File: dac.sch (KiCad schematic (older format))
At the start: 21 parts, among them J1 RCJ-2121, J2 Conn_01x03_Male, SW1 SW_DIP_x01, U1 pcm5102a

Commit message: correcciones en el esquematico indicadas  por el profesor
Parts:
- J1: Número de cátalogo (none) -> CP-1430-ND
- SW1: Código de catálogo en Digikey. (none) -> EG5071-ND
- U1: Código de catálogo en Digikey. (none) -> 296-36705-2-ND
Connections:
- net labels added: FLT, GND, OUTL, OUTR
- net labels removed: Earth
- wire segments 81 -> 77
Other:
- note added: "Conexiones del CI"
- note added: "output circuit"
- moved on the sheet: C1, C10, C11, C12, C13, C2, C3, C4, C5, C6, C7, C8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

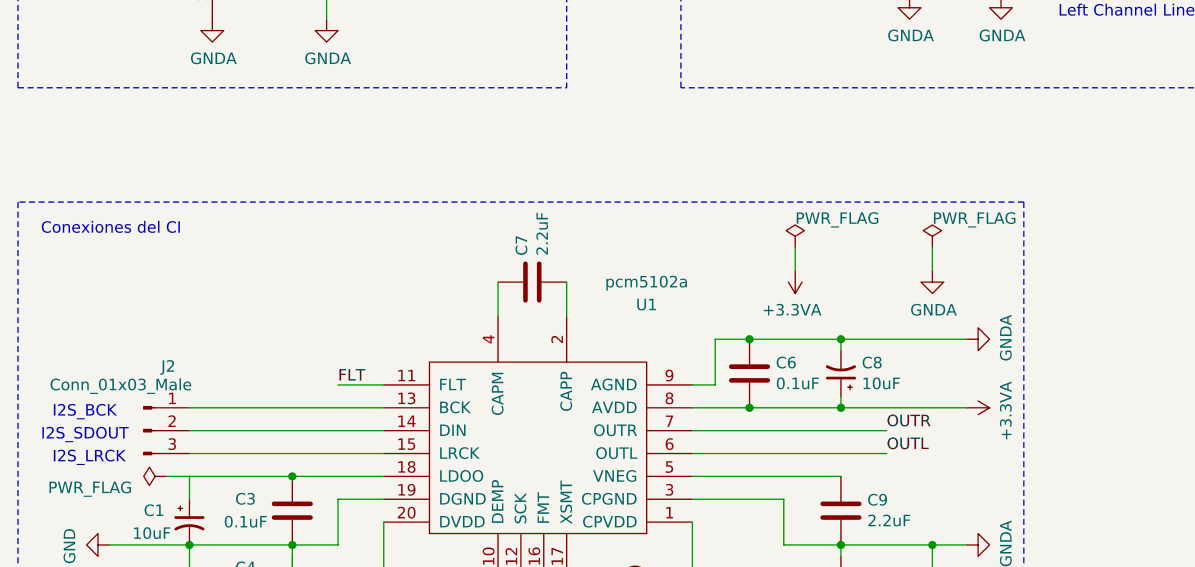
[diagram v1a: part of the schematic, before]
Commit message: pcb terminado
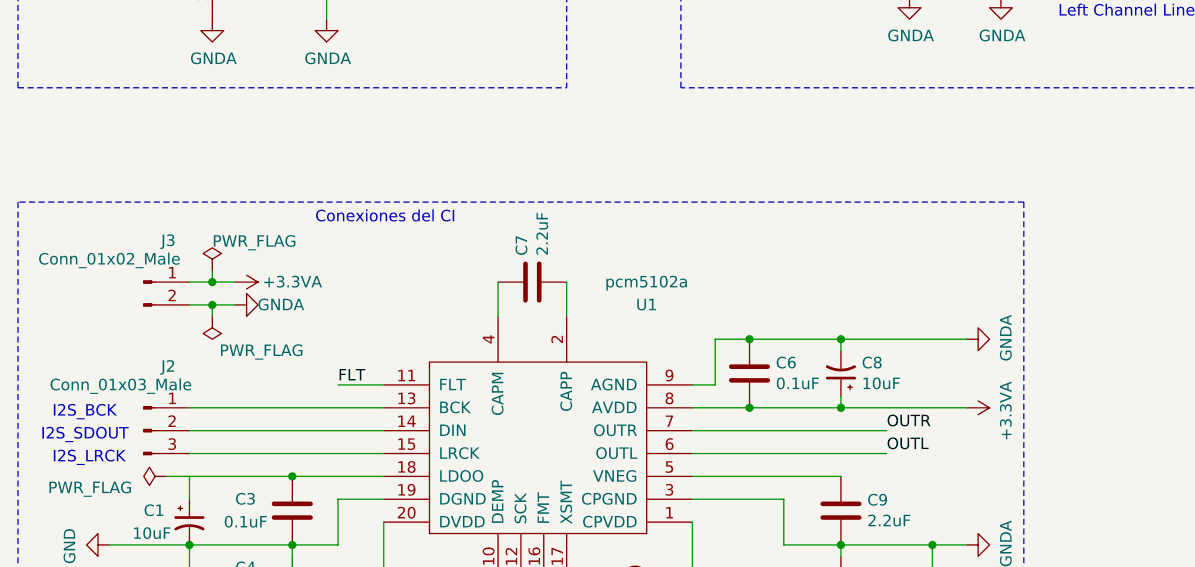
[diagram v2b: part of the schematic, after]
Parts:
- added J3: Conn_01x02_Male, Connector_PinHeader_2.54mm:PinHeader_1x02_P2.54mm_Vertical, symbol Connector:Conn_01x02_Male
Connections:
- net +3.3VA: now also J3.1 (Pin_1)
- net GNDA: now also J3.2 (Pin_2)
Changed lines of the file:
@@
 Wire Wire Line
 	6550 4150 6550 4350
-Text Notes 3600 3700 0    50   ~ 0
+Text Notes 4800 3650 0    50   ~ 0
 Conexiones del CI
 Wire Wire Line
@@
 Wire Wire Line
 	5750 5400 5750 5300
+Wire Wire Line
+	4850 2150 5200 2150
+Wire Notes Line
+	3500 3050 5900 3050
+Wire Notes Line
+	3500 1600 5900 1600
+$Comp
+L power:+3.3VA #PWR0104
+U 1 1 60A48341
+P 4450 3900
+F 0 "#PWR0104" H 4450 3750 50  0001 C CNN
+F 1 "+3.3VA" V 4450 4150 50  0000 C CNN
+F 2 "" H 4450 3900 50  0001 C CNN
+F 3 "" H 4450 3900 50  0001 C CNN
+	1    4450 3900
+	0    1    1    0
+$EndComp
+$Comp
+L power:PWR_FLAG #FLG0101
+U 1 1 60790EFD
+P 4350 3850
+F 0 "#FLG0101" H 4350 3925 50  0001 C CNN
+F 1 "PWR_FLAG" H 4350 3978 50  0000 L CNN
+F 2 "" H 4350 3850 50  0001 C CNN
+F 3 "~" H 4350 3850 50  0001 C CNN
+	1    4350 3850
+	1    0    0    -1
+$EndComp
+$Comp
+L power:PWR_FLAG #FLG0102
+U 1 1 60A4D20D
+P 4350 4050
+F 0 "#FLG0102" H 4350 4125 50  0001 C CNN
+F 1 "PWR_FLAG" H 3950 4200 50  0000 L CNN
+F 2 "" H 4350 4050 50  0001 C CNN
+F 3 "~" H 4350 4050 50  0001 C CNN
+	1    4350 4050
+	-1   0    0    1
+$EndComp
+$Comp
+L power:GNDA #PWR0103
+U 1 1 60A3D0B2
+P 4450 4000
+F 0 "#PWR0103" H 4450 3750 50  0001 C CNN
+F 1 "GNDA" V 4450 3800 50  0000 C CNN
+F 2 "" H 4450 4000 50  0001 C CNN
+F 3 "" H 4450 4000 50  0001 C CNN
+	1    4450 4000
+	0    -1   -1   0
+$EndComp
+$Comp
+L Connector:Conn_01x02_Male J3
+U 1 1 607E48C9
+P 4050 3900
+F 0 "J3" H 4158 4081 50  0000 C CNN
+F 1 "Conn_01x02_Male" H 3900 4000 50  0000 C CNN
+F 2 "Connector_PinHeader_2.54mm:PinHeader_1x02_P2.54mm_Vertical" H 4050 3900 50  0001 C CNN
+F 3 "~" H 4050 3900 50  0001 C CNN
+	1    4050 3900
+	1    0    0    -1
+$EndComp
+Wire Wire Line
+	4250 3900 4350 3900
+Wire Wire Line
+	4250 4000 4350 4000
+Wire Wire Line
+	4350 3850 4350 3900
+Connection ~ 4350 3900
+Wire Wire Line
+	4350 3900 4450 3900
+Wire Wire Line
+	4350 4050 4350 4000
+Connection ~ 4350 4000
+Wire Wire Line
+	4350 4000 4450 4000
 $Comp
 L power:PWR_FLAG #FLG0104
@@
 Wire Wire Line
 	5650 5400 5750 5400
-Wire Wire Line
-	4850 2150 5200 2150
-Wire Notes Line
-	3500 3050 5900 3050
-Wire Notes Line
-	3500 1600 5900 1600
-Wire Wire Line
-	6900 3750 6900 3850
-$Comp
-L power:+3.3VA #PWR0104
-U 1 1 60A48341
-P 6900 3850
-F 0 "#PWR0104" H 6900 3700 50  0001 C CNN
-F 1 "+3.3VA" H 6915 4023 50  0000 C CNN
-F 2 "" H 6900 3850 50  0001 C CNN
-F 3 "" H 6900 3850 50  0001 C CNN
-	1    6900 3850
-	-1   0    0    1
-$EndComp
-$Comp
-L power:PWR_FLAG #FLG0101
-U 1 1 60790EFD
-P 6900 3750
-F 0 "#FLG0101" H 6900 3825 50  0001 C CNN
-F 1 "PWR_FLAG" H 6900 3878 50  0000 L CNN
-F 2 "" H 6900 3750 50  0001 C CNN
-F 3 "~" H 6900 3750 50  0001 C CNN
-	1    6900 3750
-	1    0    0    -1
-$EndComp
-Wire Wire Line
-	7500 3750 7500 3850
-$Comp
-L power:PWR_FLAG #FLG0102
-U 1 1 60A4D20D
-P 7500 3750
-F 0 "#FLG0102" H 7500 3825 50  0001 C CNN
-F 1 "PWR_FLAG" H 7500 3878 50  0000 L CNN
-F 2 "" H 7500 3750 50  0001 C CNN
-F 3 "~" H 7500 3750 50  0001 C CNN
-	1    7500 3750
-	1    0    0    -1
-$EndComp
-$Comp
-L power:GNDA #PWR0103
-U 1 1 60A3D0B2
-P 7500 3850
-F 0 "#PWR0103" H 7500 3600 50  0001 C CNN
-F 1 "GNDA" H 7505 3677 50  0000 C CNN
-F 2 "" H 7500 3850 50  0001 C CNN
-F 3 "" H 7500 3850 50  0001 C CNN
-	1    7500 3850
-	1    0    0    -1
-$EndComp
 $EndSCHEMATC

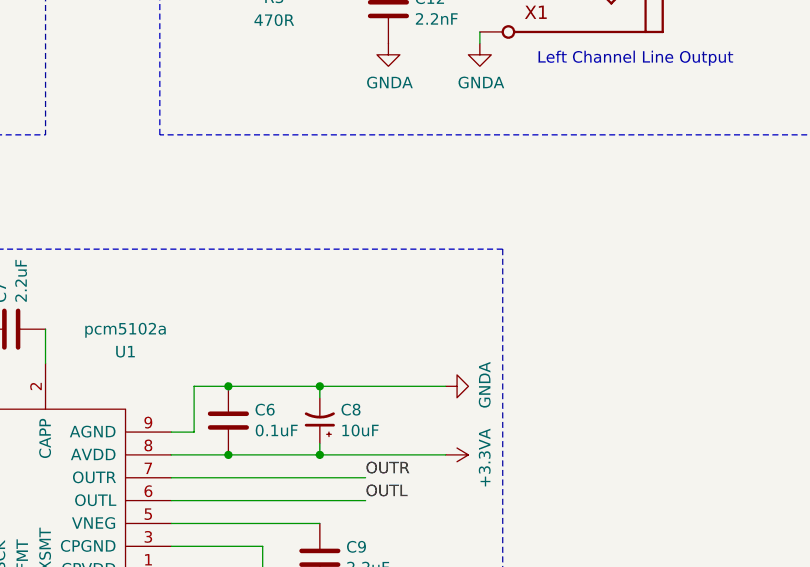
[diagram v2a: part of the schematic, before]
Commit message: correcciones pcb
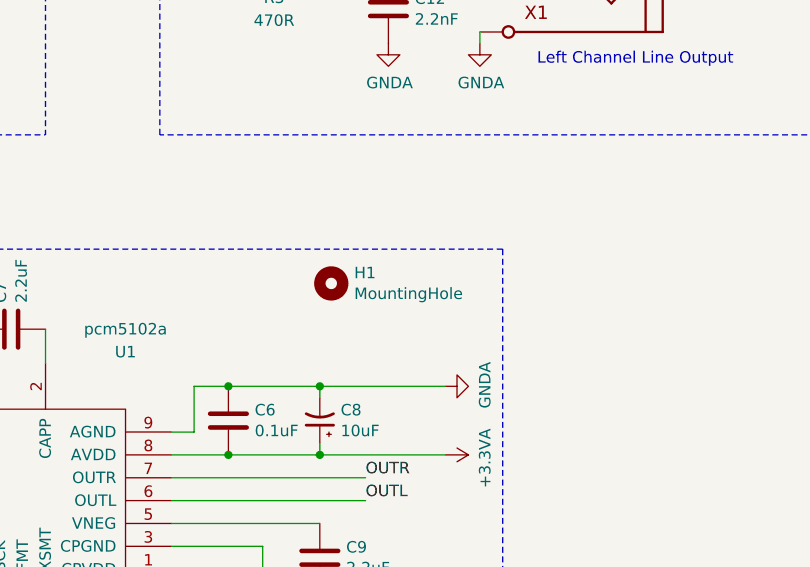
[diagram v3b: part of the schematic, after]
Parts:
- added H1: MountingHole, MountingHole:MountingHole_2.5mm, symbol Mechanical:MountingHole
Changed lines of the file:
@@
 Wire Wire Line
 	5650 5400 5750 5400
+$Comp
+L Mechanical:MountingHole H1
+U 1 1 608A30DB
+P 7150 3700
+F 0 "H1" H 7250 3746 50  0000 L CNN
+F 1 "MountingHole" H 7250 3655 50  0000 L CNN
+F 2 "MountingHole:MountingHole_2.5mm" H 7150 3700 50  0001 C CNN
+F 3 "~" H 7150 3700 50  0001 C CNN
+	1    7150 3700
+	1    0    0    -1
+$EndComp
 $EndSCHEMATC
